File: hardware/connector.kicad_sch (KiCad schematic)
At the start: 5 parts, among them J1 SAFETY_SUPPLY, J2 SWDIO_CONN, J3 SENSORS, J4 VALVES, J5 MAIN

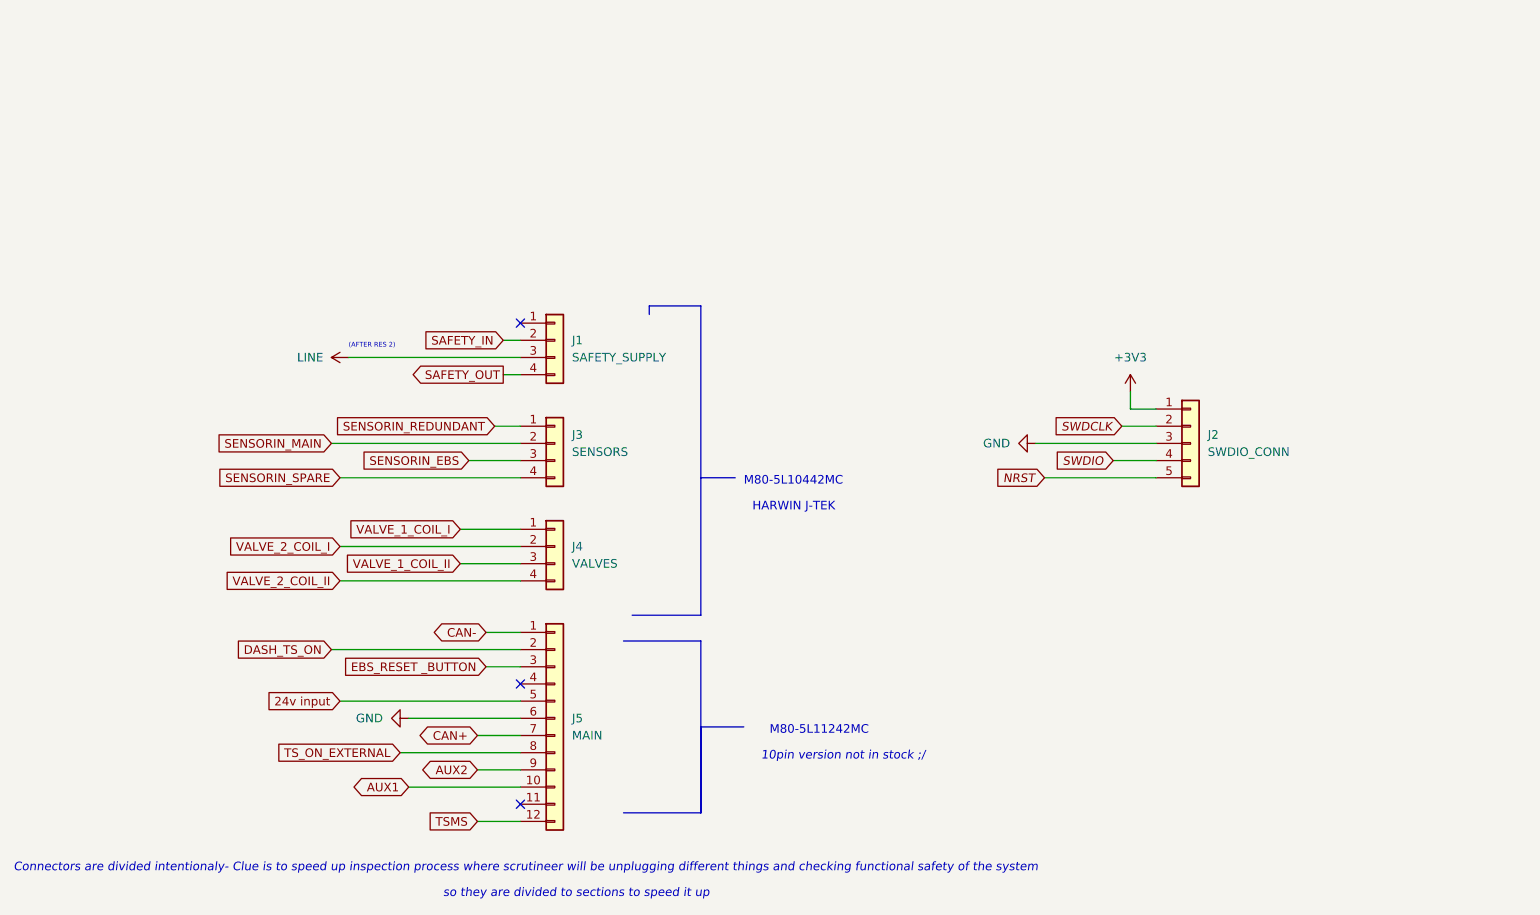
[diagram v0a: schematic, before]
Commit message: 2.0 layot wip , routing 3
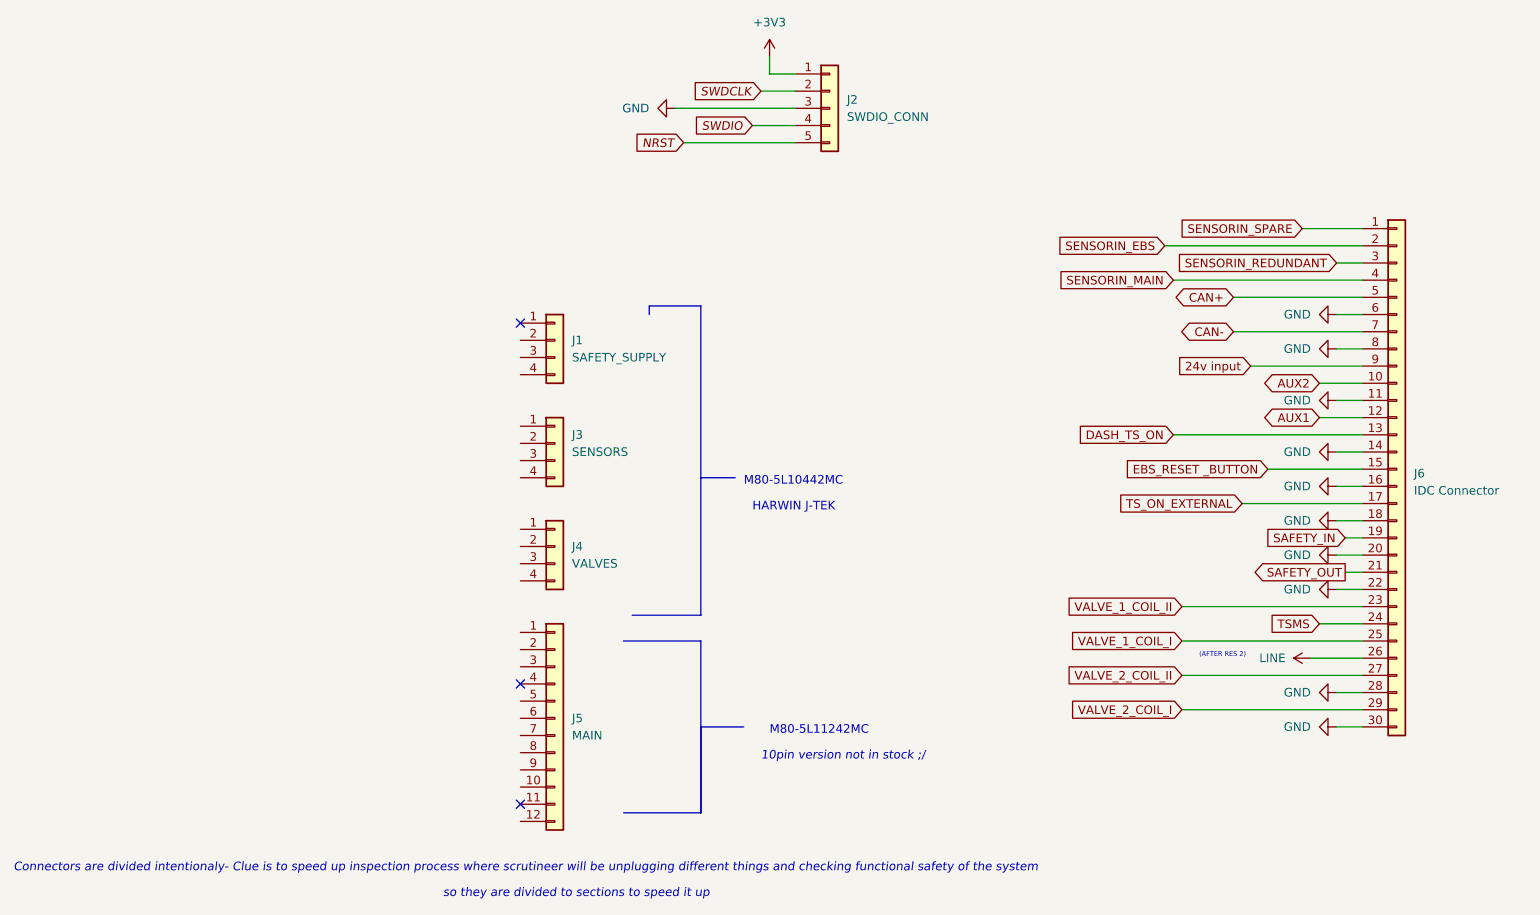
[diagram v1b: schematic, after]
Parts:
- added J6: IDC Connector, Connector_IDC:IDC-Header_2x15-1MP_P2.54mm_Latch6.5mm_Vertical, symbol Connector_Generic:Conn_01x30
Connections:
- net 24v input: now also J6.9 (Pin_9); no longer J5.5 (Pin_5)
- net AUX1: now also J6.12 (Pin_12); no longer J5.10 (Pin_10)
- net AUX2: now also J6.10 (Pin_10); no longer J5.9 (Pin_9)
- net CAN+: now also J6.5 (Pin_5); no longer J5.7 (Pin_7)
- net CAN-: now also J6.7 (Pin_7); no longer J5.1 (Pin_1)
- net DASH_TS_ON: now also J6.13 (Pin_13); no longer J5.2 (Pin_2)
- net EBS_RESET _BUTTON: now also J6.15 (Pin_15); no longer J5.3 (Pin_3)
- net GND: now also J6.11 (Pin_11), J6.14 (Pin_14), J6.16 (Pin_16), J6.18 (Pin_18), J6.20 (Pin_20), J6.22 (Pin_22), J6.28 (Pin_28), J6.30 (Pin_30), J6.6 (Pin_6), J6.8 (Pin_8); no longer J5.6 (Pin_6)
- net LINE: now also J6.26 (Pin_26); no longer J1.3 (Pin_3)
- net SAFETY_IN: now also J6.19 (Pin_19); no longer J1.2 (Pin_2)
- net SAFETY_OUT: now also J6.21 (Pin_21); no longer J1.4 (Pin_4)
- net SENSORIN_EBS: now also J6.2 (Pin_2); no longer J3.3 (Pin_3)
- net SENSORIN_MAIN: now also J6.4 (Pin_4); no longer J3.2 (Pin_2)
- net SENSORIN_REDUNDANT: now also J6.3 (Pin_3); no longer J3.1 (Pin_1)
- net SENSORIN_SPARE: now also J6.1 (Pin_1); no longer J3.4 (Pin_4)
- net TSMS: now also J6.24 (Pin_24); no longer J5.12 (Pin_12)
- net TS_ON_EXTERNAL: now also J6.17 (Pin_17); no longer J5.8 (Pin_8)
- net VALVE_1_COIL_I: now also J6.25 (Pin_25); no longer J4.1 (Pin_1)
- net VALVE_1_COIL_II: now also J6.23 (Pin_23); no longer J4.3 (Pin_3)
- net VALVE_2_COIL_I: now also J6.29 (Pin_29); no longer J4.2 (Pin_2)
- net VALVE_2_COIL_II: now also J6.27 (Pin_27); no longer J4.4 (Pin_4)
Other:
- moved on the sheet: J2
